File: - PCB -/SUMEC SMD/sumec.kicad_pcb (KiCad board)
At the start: 2 copper layers, 92 x 84 mm, 55 parts, among them IC1 XT30U-F, J1 Conn_01x04_Pin, J2 USB3090-XX-X_REVE, J3 Conn_01x06_Pin, J4 Conn_01x06_Pin, J5 Conn_01x06_Pin, J6 Conn_01x01_Pin, J8 Conn_01x03_Pin, Q1 PMOS, SW1 SW_SPDT, SW2 SW_Push, SW3 SW_Push, SW4 SW_Push, U1 TB6612FNG, U11 LM1084-3.3, U12 QRE1113, U13 QRE1113, U5 TSOP382xx, U6 QRE1113, U7 QRE1113, U9 ESP32-S3-WROOM-1

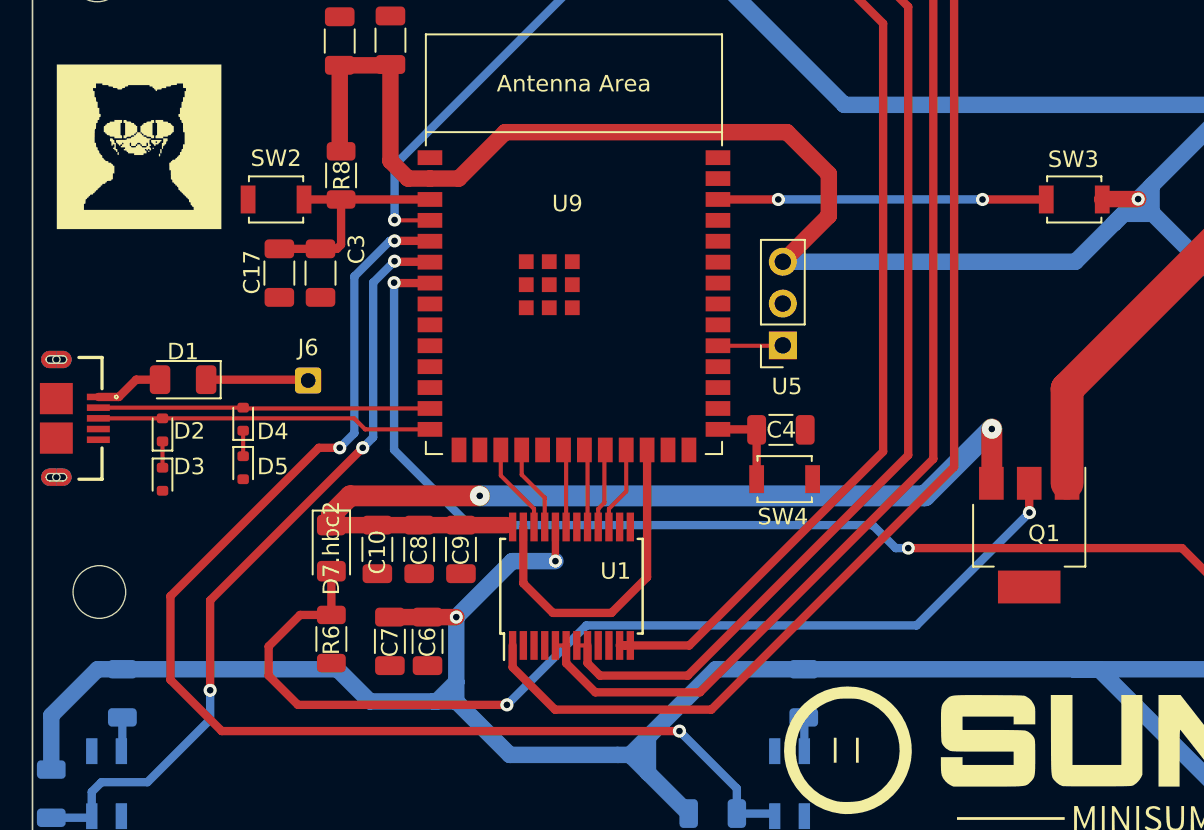
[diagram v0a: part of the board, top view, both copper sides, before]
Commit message: pcb board update
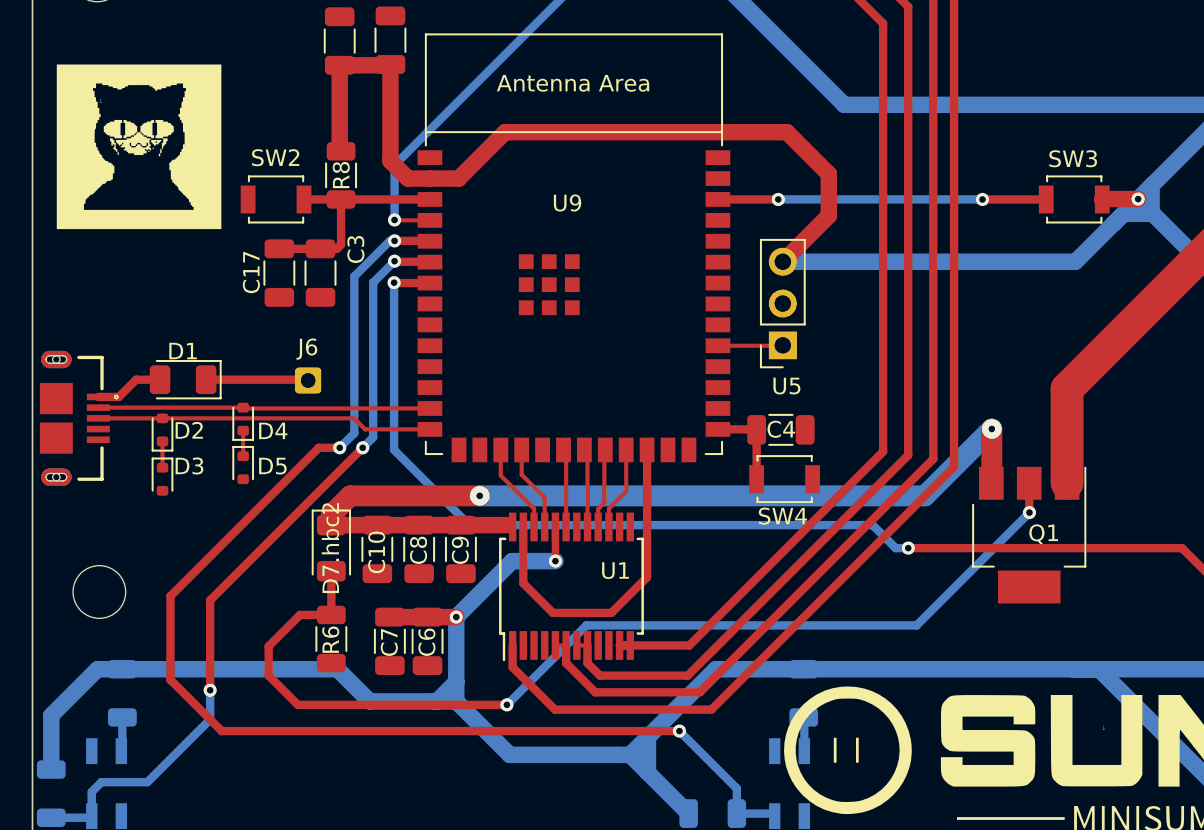
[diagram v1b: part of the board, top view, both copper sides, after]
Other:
- board text added: ">:3"
